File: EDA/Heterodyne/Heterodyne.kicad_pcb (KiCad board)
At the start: 4 copper layers, 35.5 x 19 mm, 43 parts, among them J1 Conn_01x06, J7 Reciever, U1 SA612AD, U2 OPA2830, U3 MAX7375AXR105, U4 MAX11613, U5 ATmega328PB-AU, Y1 8 MHz

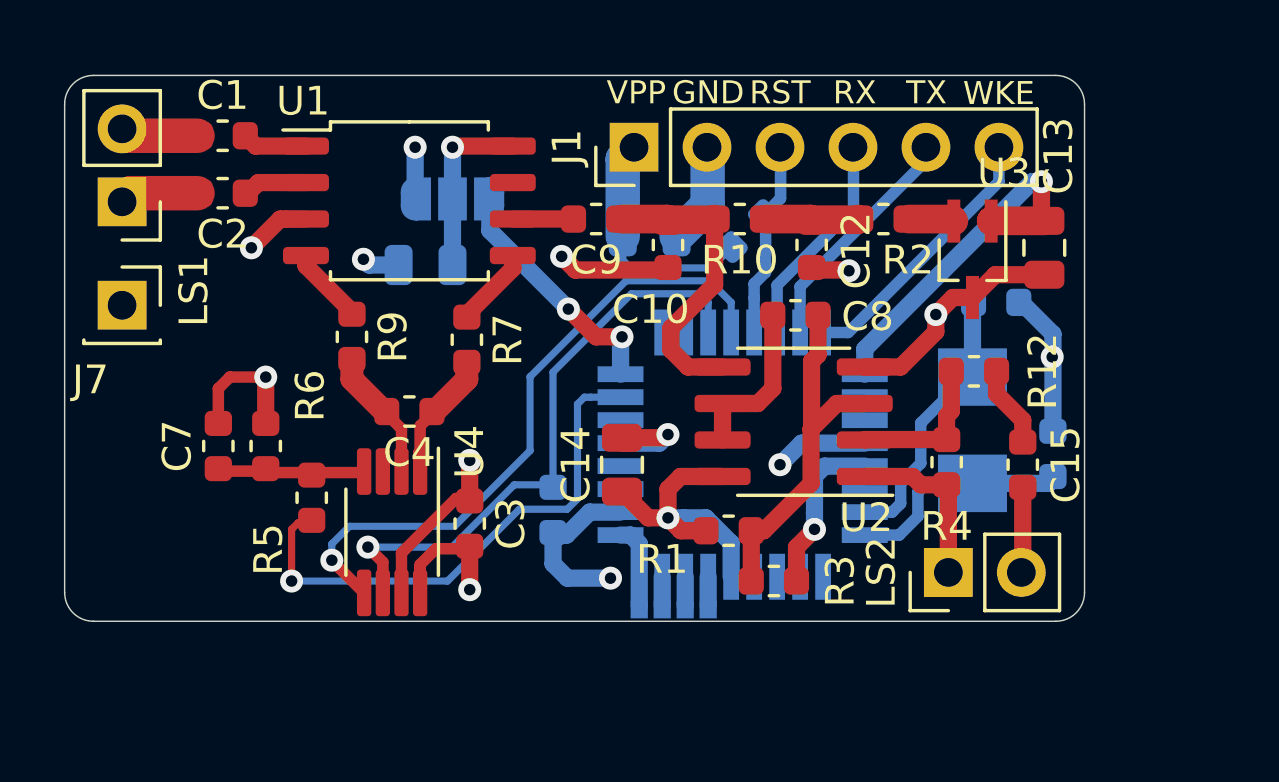
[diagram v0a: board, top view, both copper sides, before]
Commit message: initial commit of SAMD21 branch
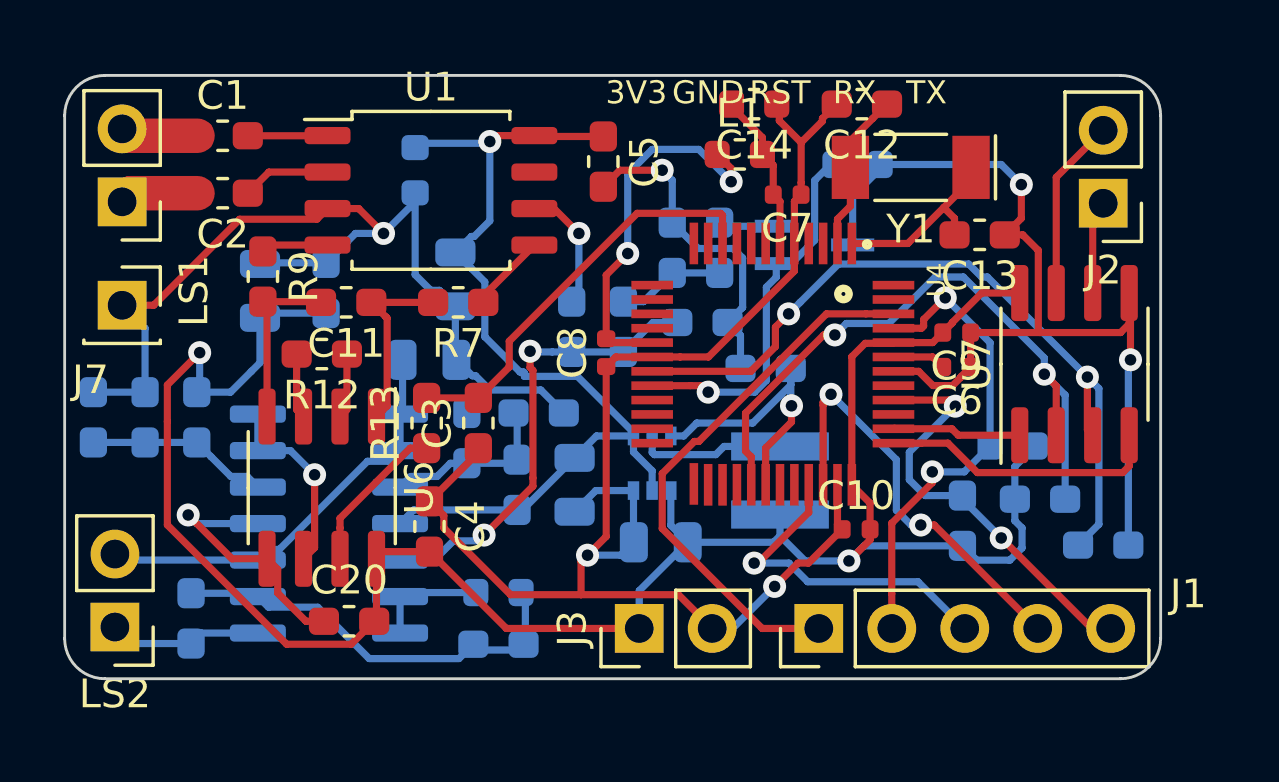
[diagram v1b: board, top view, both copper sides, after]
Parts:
- removed JP1: SolderJumper_3_Open, Jumper:SolderJumper-3_P1.3mm_Open_RoundedPad1.0x1.5mm_NumberLabels
- removed TP1, TP2, TP3, TP4: TestPoint, Heterodyne:Testpoint SPI
- added C17: 330 pF, Capacitor_SMD:C_0603_1608Metric_Pad1.05x0.95mm_HandSolder, B.Cu at (121.2, 55.8)
- added C18: 3.3 μF, Capacitor_SMD:C_0805_2012Metric, B.Cu at (110.3, 54.5)
- added C19: 1 uF, Capacitor_SMD:C_0603_1608Metric_Pad1.05x0.95mm_HandSolder, B.Cu at (104.5, 58.9)
- added C20: 1 uF, Capacitor_SMD:C_0603_1608Metric_Pad1.05x0.95mm_HandSolder, F.Cu at (113.4, 66.0)
- added C21: 1 uF, Capacitor_SMD:C_0603_1608Metric_Pad1.05x0.95mm_HandSolder, B.Cu at (112.6, 54.4)
- added C22: 1 μF, Capacitor_SMD:C_0603_1608Metric_Pad1.05x0.95mm_HandSolder, B.Cu at (117.5, 59.6)
- added C22: 2.2 μF, Capacitor_SMD:C_0805_2012Metric, B.Cu at (117.1, 54.1)
- added C23: 1 μF, Capacitor_SMD:C_0603_1608Metric, B.Cu at (131.1, 50.1)
- added C24: 1 μF, Capacitor_SMD:C_0603_1608Metric, B.Cu at (115.7, 50.3)
- added C25: 1 μF, Capacitor_SMD:C_0603_1608Metric, B.Cu at (118.6, 65.0)
- added C26: 10 μF, Capacitor_SMD:C_0805_2012Metric, B.Cu at (124.2, 63.2)
- added C27: 10 μF, Capacitor_SMD:C_0805_2012Metric, B.Cu at (116.2, 56.9)
- added C28: 10 μF, Capacitor_SMD:C_0805_2012Metric, B.Cu at (121.2, 61.2)
- added J2: Conn_01x02, Connector_PinHeader_2.54mm:PinHeader_1x02_P2.54mm_Vertical, F.Cu at (139.7, 51.5)
- added J3: Conn_01x02, Connector_PinHeader_2.54mm:PinHeader_1x02_P2.54mm_Vertical, F.Cu at (123.5, 66.2)
- added L1: BLM18PG471SN1D, Capacitor_SMD:C_0603_1608Metric, F.Cu at (127.0, 49.8)
- added L2: XFL4020-472MEC, Inductor_SMD:L_Coilcraft_XxL4020, B.Cu at (128.4, 61.1)
- added R13: 100 Ω, Resistor_SMD:R_0603_1608Metric_Pad1.05x0.95mm_HandSolder, F.Cu at (116.1, 59.1)
- added R14: 10 kΩ, Resistor_SMD:R_0603_1608Metric_Pad1.05x0.95mm_HandSolder, B.Cu at (119.2, 61.2)
- added R15: 10 kΩ, Resistor_SMD:R_0603_1608Metric_Pad1.05x0.95mm_HandSolder, B.Cu at (120.0, 58.8)
- added R16: 1 kΩ, Resistor_SMD:R_0603_1608Metric_Pad1.05x0.95mm_HandSolder, B.Cu at (118.6, 66.8)
- added R17: 15 kΩ, Resistor_SMD:R_0603_1608Metric_Pad1.05x0.95mm_HandSolder, B.Cu at (107.9, 65.9)
- added U6: AD8226, Package_SO:SOIC-8_3.9x4.9mm_P1.27mm, F.Cu at (112.5, 61.4)
- added U7: SP3075, Package_SO:SOIC-8_3.9x4.9mm_P1.27mm, F.Cu at (138.7, 57.0)
- C1, C2, C3: footprint Capacitor_SMD:C_0603_1608Metric -> Capacitor_SMD:C_0603_1608Metric_Pad1.05x0.95mm_HandSolder
- C10, C9: value 330 pF -> 100 nF; footprint Capacitor_SMD:C_0603_1608Metric -> Capacitor_SMD:C_0402_1005Metric
- C11: value 3.3 μF -> 22 nF; footprint Capacitor_SMD:C_0805_2012Metric -> Capacitor_SMD:C_0603_1608Metric_Pad1.05x0.95mm_HandSolder; moved to F.Cu
- C12: value 330 pF -> 18 pF; footprint Capacitor_SMD:C_0603_1608Metric -> Capacitor_SMD:C_0603_1608Metric_Pad1.05x0.95mm_HandSolder
- C13: value 3.3 μF -> 18 pF; footprint Capacitor_SMD:C_0805_2012Metric -> Capacitor_SMD:C_0603_1608Metric_Pad1.05x0.95mm_HandSolder
- C14: value 3.3 μF -> 4.7uF; footprint Capacitor_SMD:C_0805_2012Metric -> Capacitor_SMD:C_0603_1608Metric
- C15: value 1 nF -> 330 pF; footprint Capacitor_SMD:C_0603_1608Metric -> Capacitor_SMD:C_0603_1608Metric_Pad1.05x0.95mm_HandSolder; moved to B.Cu
- C16: value 3.3 μF -> 330 pF; footprint Capacitor_SMD:C_0805_2012Metric -> Capacitor_SMD:C_0603_1608Metric_Pad1.05x0.95mm_HandSolder
- C4: value 22 nF -> 100 nF; footprint Capacitor_SMD:C_0603_1608Metric -> Capacitor_SMD:C_0603_1608Metric_Pad1.05x0.95mm_HandSolder
- C5: value 18 pF -> 100 nF; footprint Capacitor_SMD:C_0603_1608Metric -> Capacitor_SMD:C_0603_1608Metric_Pad1.05x0.95mm_HandSolder; moved to F.Cu
- C6: value 18 pF -> 100 nF; footprint Capacitor_SMD:C_0603_1608Metric -> Capacitor_SMD:C_0402_1005Metric; moved to F.Cu
- C7: footprint Capacitor_SMD:C_0603_1608Metric -> Capacitor_SMD:C_0402_1005Metric
- C8: value 1 nF -> 100 nF; footprint Capacitor_SMD:C_0603_1608Metric -> Capacitor_SMD:C_0402_1005Metric
- J1: value Conn_01x06 -> Conn_01x05; footprint Connector_PinHeader_2.54mm:PinHeader_1x06_P2.54mm_Vertical -> Connector_PinHeader_2.54mm:PinHeader_1x05_P2.54mm_Vertical
- R1, R3: value 1 kΩ -> 20 kΩ; footprint Resistor_SMD:R_0603_1608Metric -> Resistor_SMD:R_0603_1608Metric_Pad1.05x0.95mm_HandSolder; moved to B.Cu
- R10, R2: footprint Resistor_SMD:R_0603_1608Metric -> Resistor_SMD:R_0603_1608Metric_Pad1.05x0.95mm_HandSolder; moved to B.Cu
- R11: value 10 kΩ -> 500 kΩ; footprint Resistor_SMD:R_0603_1608Metric -> Resistor_SMD:R_0603_1608Metric_Pad1.05x0.95mm_HandSolder
- R12: value 1 kΩ -> 200 Ω; footprint Resistor_SMD:R_0603_1608Metric -> Resistor_SMD:R_0603_1608Metric_Pad1.05x0.95mm_HandSolder
- R4: value 12 kΩ -> 10 kΩ; footprint Resistor_SMD:R_0603_1608Metric -> Resistor_SMD:R_0603_1608Metric_Pad1.05x0.95mm_HandSolder; moved to B.Cu
- R5: value 10 kΩ -> 1 kΩ; moved to B.Cu
- R6: value 1 kΩ -> 2.8 MΩ; footprint Resistor_SMD:R_0603_1608Metric -> Resistor_SMD:R_0603_1608Metric_Pad1.05x0.95mm_HandSolder; moved to B.Cu
- R7, R8, R9: footprint Resistor_SMD:R_0603_1608Metric -> Resistor_SMD:R_0603_1608Metric_Pad1.05x0.95mm_HandSolder
- U2: value OPA2830 -> OPA4354; footprint Package_SO:SOIC-8_3.9x4.9mm_P1.27mm -> Package_SO:SOIC-14_3.9x8.7mm_P1.27mm; moved to B.Cu
- U3: moved to B.Cu
- U4: value MAX11613 -> ATSAMD21G18A-AUT; footprint Package_SO:MSOP-8_3x3mm_P0.65mm -> ATSAMD21G18A-AUT:QFP50P900X900X120-48N
- U5: value ATmega328PB-AU -> TPS61222; footprint Package_QFP:TQFP-32_7x7mm_P0.8mm -> Package_TO_SOT_SMD:SOT-363_SC-70-6
- Y1: value 8 MHz -> FX255_32.768kHz; footprint Crystal:Crystal_SMD_5032-2Pin_5.0x3.2mm -> Crystal:Crystal_SMD_MicroCrystal_CC4V-T1A-2Pin_5.0x1.9mm; moved to F.Cu
- moved LS2 29.1 mm to (105.2, 66.2), turned to 180 degrees
- moved R5 24.5 mm to (136.5, 59.9), turned to 0 degrees
- moved R12 22.7 mm to (112.5, 56.7)
- moved C7 21.6 mm to (128.7, 51.1), turned to 180 degrees
- moved J1 17.9 mm to (129.8, 66.2)
- moved U2 16.6 mm to (112.7, 62.6)
- moved R11 14.6 mm to (106.3, 58.9), turned to 90 degrees
- moved C5 14.5 mm to (122.2, 50.0), turned to 270 degrees
- moved U4 14.5 mm to (128.2, 57.0)
- moved C15 14.3 mm to (124.7, 53.0)
- moved C14 13.4 mm to (127.5, 48.0), turned to 180 degrees
- moved C9 13.2 mm to (134.6, 56.0)
- moved R8 12.5 mm to (134.8, 62.5), turned to 270 degrees
- moved C10 11.9 mm to (131.1, 62.8), turned to 0 degrees
- moved R3 11.5 mm to (139.7, 63.4), turned to 0 degrees
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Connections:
- C10 pad 2: Driver_Wave -> +3V3
- C11 pad 1: VPP -> Net-(C11-Pad1)
- C11 pad 2: GND -> Net-(C11-Pad2)
- C13 pad 2: VCLOCK -> Net-(C13-Pad2)
- C14 pad 1: VOPAMP -> GND
- C14 pad 2: GND -> Net-(C14-Pad2)
- C15 pad 1: GND -> Net-(C15-Pad1)
- C15 pad 2: Net-(C15-Pad2) -> GND
- C16 pad 2: Net-(C16-Pad2) -> Driver_Wave
- C3 pad 2: VPP -> ADC_DIFF
- C4 pad 1: Net-(C4-Pad1) -> GND
- C4 pad 2: Net-(C4-Pad2) -> +3V3
- C5 pad 1: GND -> +5V
- C5 pad 2: Net-(C5-Pad2) -> GND
- C6 pad 1: Net-(C6-Pad1) -> GND
- C6 pad 2: GND -> Net-(C6-Pad2)
- C7 pad 1: Net-(C7-Pad1) -> GND
- C7 pad 2: GND -> Net-(C14-Pad2)
- C8 pad 1: Net-(C8-Pad1) -> GND
- C8 pad 2: Net-(C8-Pad2) -> +3V3
- C9 pad 1: Driver_Wave -> GND
- C9 pad 2: Net-(C9-Pad2) -> +3V3
- J1 pad 1: VPP -> SWDIO
- J1 pad 2: GND -> SWCLK
- J1 pad 3: TTL_RST -> USB_D-
- J1 pad 4: TTL_RX -> USB_D+
- J1 pad 5: TTL_TX -> TTL_RST
- LS2 pad 2: GND -> Net-(C27-Pad2)
- R1 pad 1: VOPAMP -> +3V3
- R1 pad 2: Net-(C8-Pad2) -> RS485_RE
- R10 pad 1: Net-(C12-Pad1) -> Net-(C15-Pad1)
- R11 pad 1: SDA -> Net-(C19-Pad2)
- R11 pad 2: VPP -> GND
- R12 pad 1: Net-(C15-Pad2) -> Net-(R12-Pad1)
- R2 pad 2: Net-(C12-Pad1) -> Net-(C15-Pad1)
- R3 pad 1: GND -> RS485_DE
- R3 pad 2: Net-(C8-Pad2) -> GND
- R4 pad 1: Net-(R12-Pad2) -> BUCK_EN
- R4 pad 2: Net-(LS2-Pad1) -> GND
- R5 pad 1: VREF -> SWCLK
- R5 pad 2: Net-(C7-Pad1) -> +3V3
- R6 pad 1: Net-(C7-Pad1) -> +3V3
- R6 pad 2: GND -> Net-(C19-Pad2)
- R7 pad 2: Net-(C4-Pad1) -> Net-(C11-Pad1)
- R8 pad 1: VPP -> TTL_RST
- R8 pad 2: TTL_RST -> +3V3
- R9 pad 2: Net-(C4-Pad2) -> Net-(C11-Pad2)
- U1 pad 6: Net-(C9-Pad2) -> Net-(C17-Pad2)
- U1 pad 8: Net-(C16-Pad2) -> +5V
- U2 pad 1: Net-(LS2-Pad1) -> Net-(C27-Pad2)
- U2 pad 2: Net-(R12-Pad2) -> Net-(C27-Pad2)
- U2 pad 3: Net-(C8-Pad2) -> Net-(C22-Pad2)
- U2 pad 4: GND -> +5V
- U2 pad 6: Net-(C8-Pad1) -> Net-(C25-Pad1)
- U2 pad 7: Net-(C8-Pad1) -> Net-(C25-Pad1)
- U2 pad 8: VOPAMP -> Net-(LS2-Pad1)
- U4 pad 1: Net-(C4-Pad1) -> Net-(C13-Pad2)
- U4 pad 2: Net-(C4-Pad2) -> Net-(C12-Pad1)
- U4 pad 4: Net-(C7-Pad1) -> VREF
- U4 pad 5: SCL -> GND
- U4 pad 6: SDA -> Net-(C14-Pad2)
- U4 pad 7: GND -> Net-(U4-Pad7)
- U4 pad 8: VPP -> Net-(U4-Pad8)
- U5 pad 1: VCLOCK -> +3V3
- U5 pad 2: Net-(U5-Pad2) -> +5V
- U5 pad 3: Net-(U5-Pad3) -> GND
- U5 pad 4: VPP -> +5V
- U5 pad 5: GND -> Net-(L2-Pad2)
- U5 pad 6: Net-(U5-Pad6) -> BUCK_EN
- Y1 pad 1: Net-(C5-Pad2) -> Net-(C13-Pad2)
- Y1 pad 2: Net-(C6-Pad1) -> Net-(C12-Pad1)
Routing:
- net GND: track 47.7 -> 142.5 mm, vias 10 -> 7
- net +3V3: track 0.00 -> 87.4 mm, vias 0 -> 4
- net +5V: track 0.00 -> 32.8 mm, vias 0 -> 1
- net RS485_DE: track 0.00 -> 27.1 mm, vias 0 -> 2
- net VPP: track 24.4 -> 0.00 mm, vias 4 -> 0
- net RS485_RE: track 0.00 -> 23.6 mm, vias 0 -> 2
- net SCL: track 22.7 -> 0.00 mm, vias 1 -> 0
- net SDA: track 20.8 -> 0.00 mm, vias 1 -> 0
- net SWDIO: track 0.00 -> 19.2 mm
- net VREF: track 18.6 -> 0.00 mm, vias 1 -> 0
- net SWCLK: track 0.00 -> 16.6 mm, vias 0 -> 2
- net Net-(C27-Pad2): track 0.00 -> 15.1 mm
- net USB_D+: track 0.00 -> 15.0 mm, vias 0 -> 2
- net ADC_DIFF: track 0.00 -> 14.5 mm
- net Net-(C8-Pad2): track 12.7 -> 0.00 mm
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- added copper zone on In2.Cu, net +3V3
- removed copper zone on In2.Cu, net VPP
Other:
- board size 35.5 x 19 mm -> 38.2 x 21 mm
- board text added: "3V3"
- board text added: "BoSL Velocity Rev 0.2"
- board text removed: "BoSL Velocity rev 0.1.3"
- board text removed: "CLOSE 3 AT MANUFATURE"
- board text removed: "VPP"
- board text removed: "WKE"
